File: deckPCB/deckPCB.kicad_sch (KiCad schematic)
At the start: 29 parts, among them J1 USB_C_Receptacle_USB2.0_16P, J2 Conn_01x06_Pin, SW1 SW_Push, SW10 SW_Push, SW11 SW_Push, SW12 SW_Push, SW13 SW_Push, SW14 SW_Push, SW15 SW_Push, SW2 SW_Push, SW3 SW_Push, SW4 SW_Push, SW5 SW_Push, SW6 SW_Push, SW7 SW_Push, SW8 SW_Push, SW9 SW_Push, U1 RP2040, U2 W25Q128JVE, U3 IP5306, U4 AMS1117-3.3, U5 PAM8403DR, X1 DF40HC_3.0_-100DS-0.4V_58, X2 DF40HC_3.0_-100DS-0.4V_58

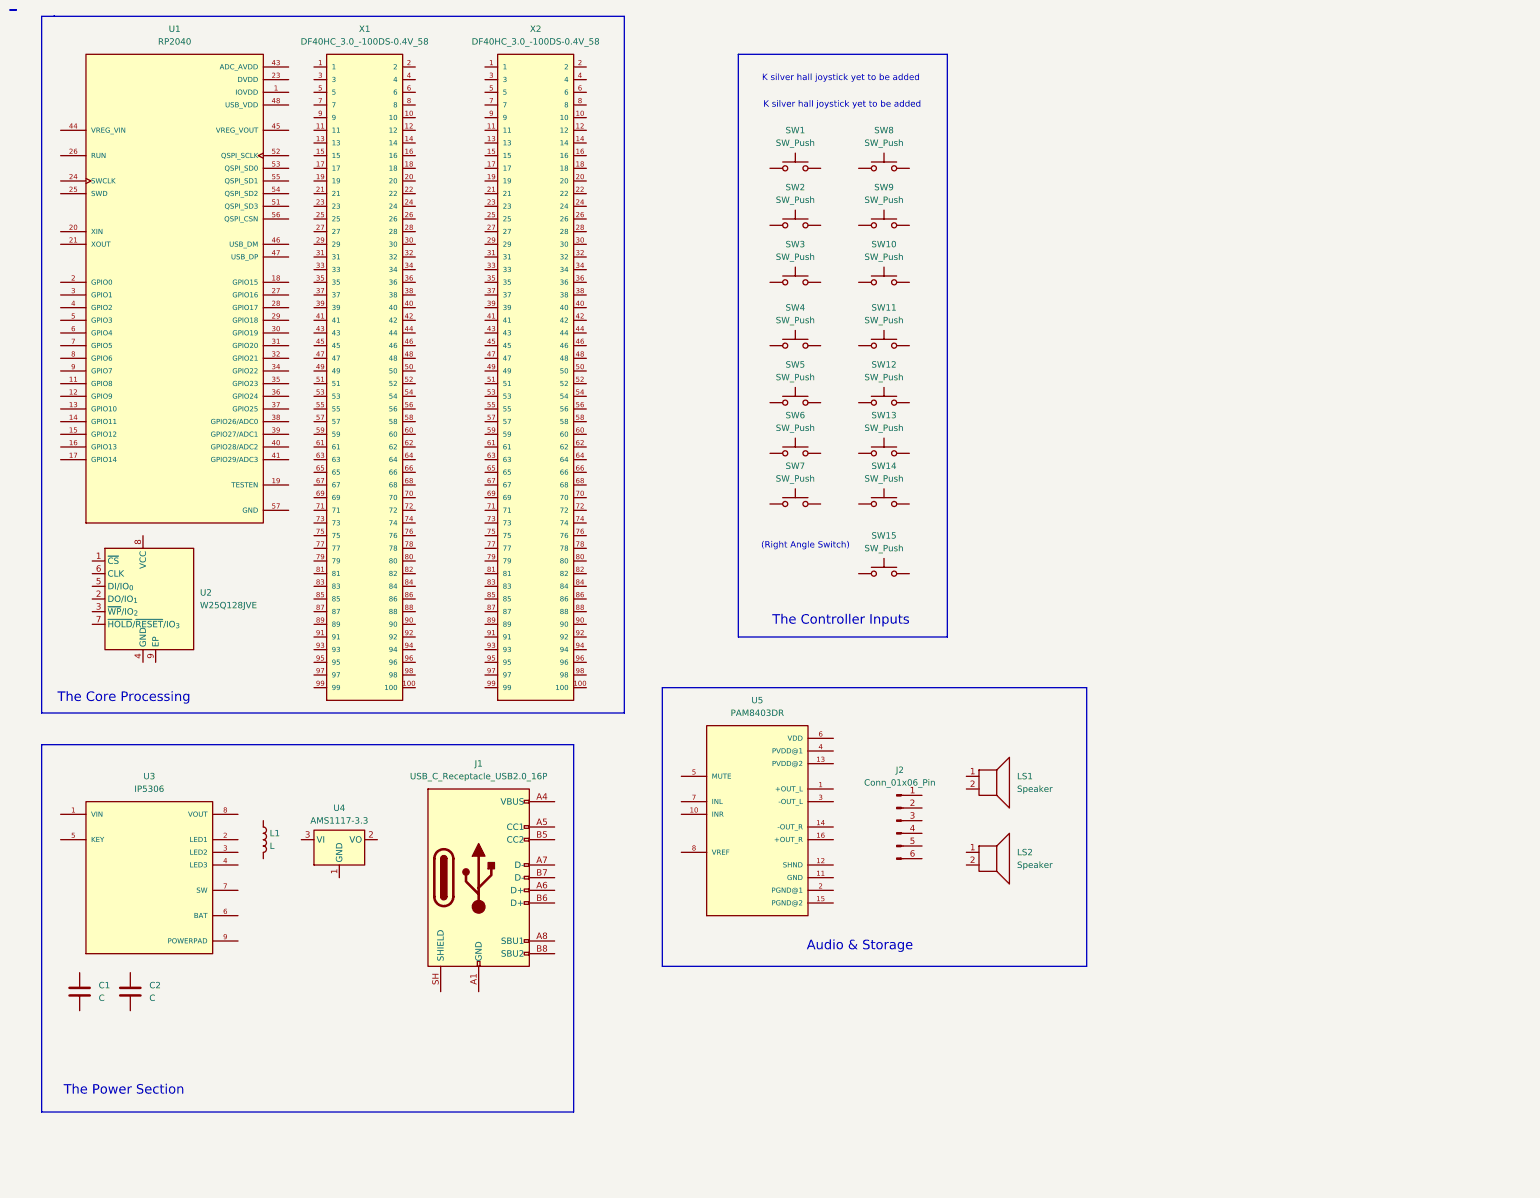
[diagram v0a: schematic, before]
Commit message: Finishing with the passives.
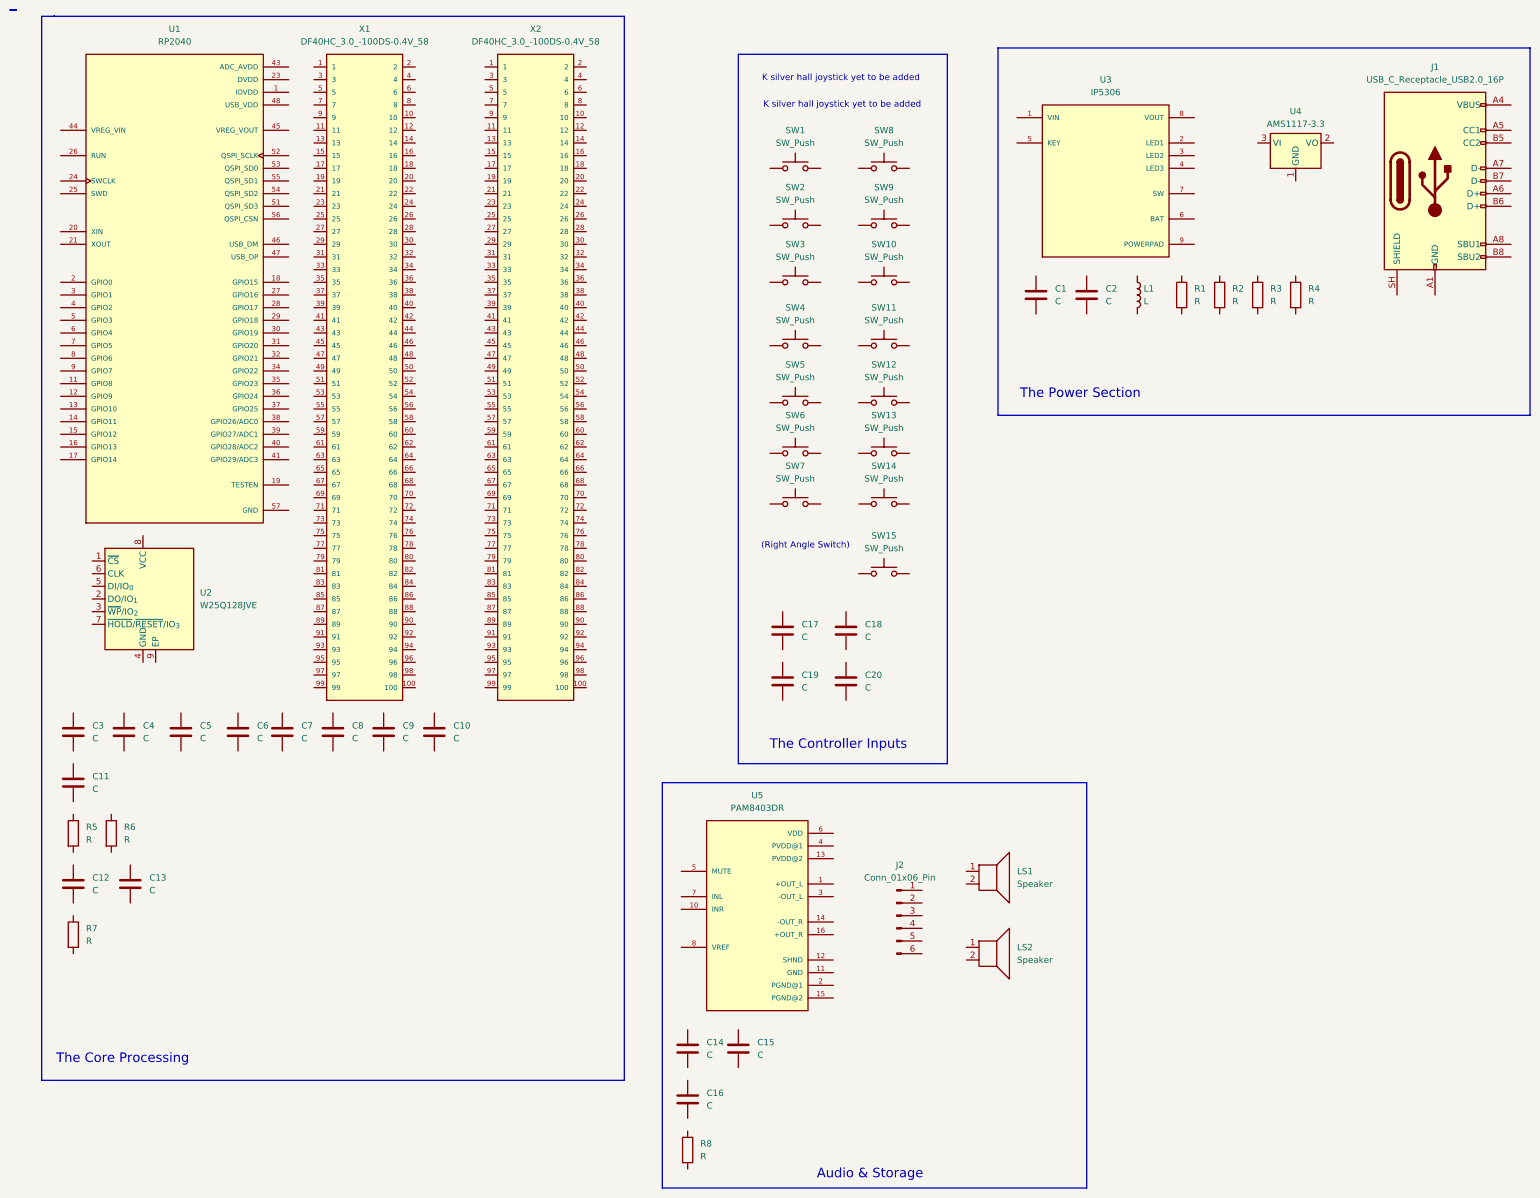
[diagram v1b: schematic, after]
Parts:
- added C10, C11, C12, C13, C14, C15, C16, C17, C18, C19, C20, C3, C4, C5, C6, C7, C8, C9: C, symbol Device:C
- added R1, R2, R3, R4, R5, R6, R7, R8: R, symbol Device:R
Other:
- moved on the sheet: C1, C2, J1, J2, L1, LS1, LS2, U3, U4, U5

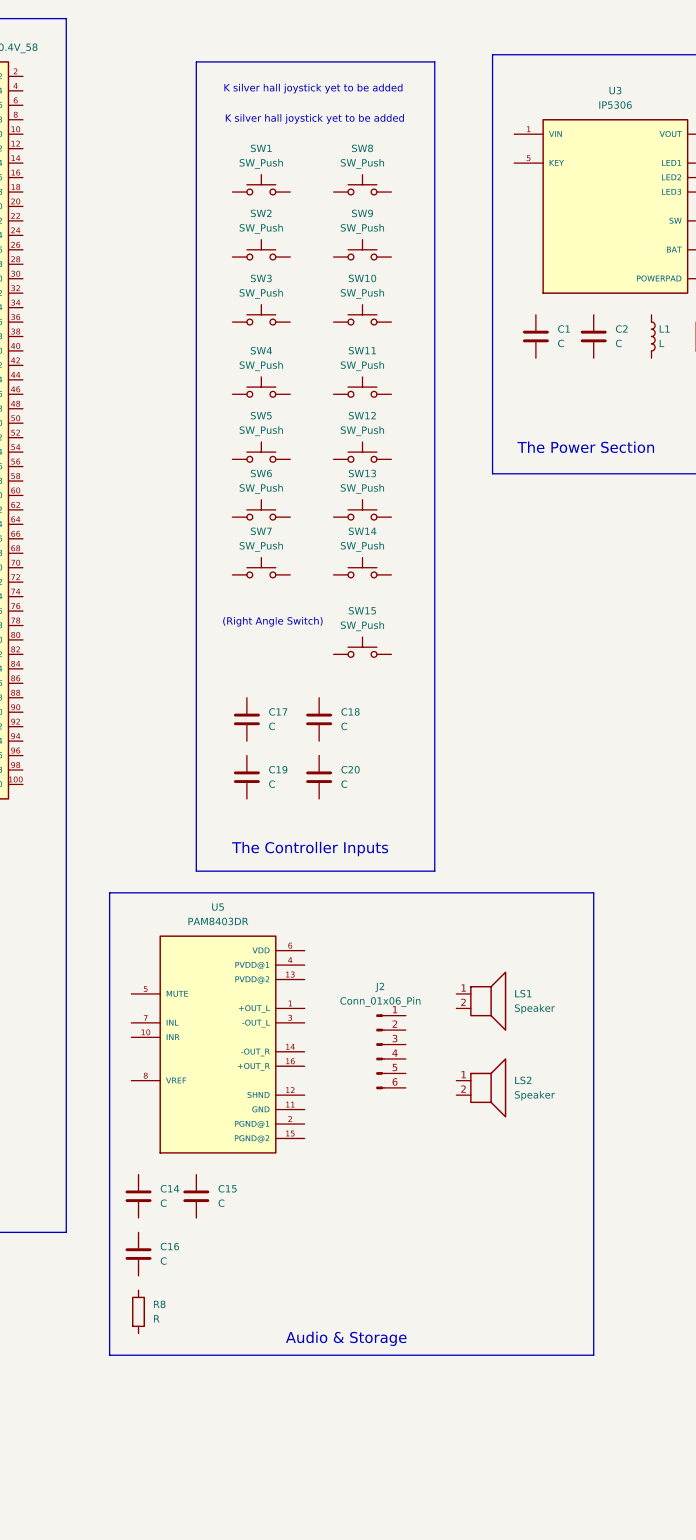
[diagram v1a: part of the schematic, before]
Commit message: hall symbol in the schematic
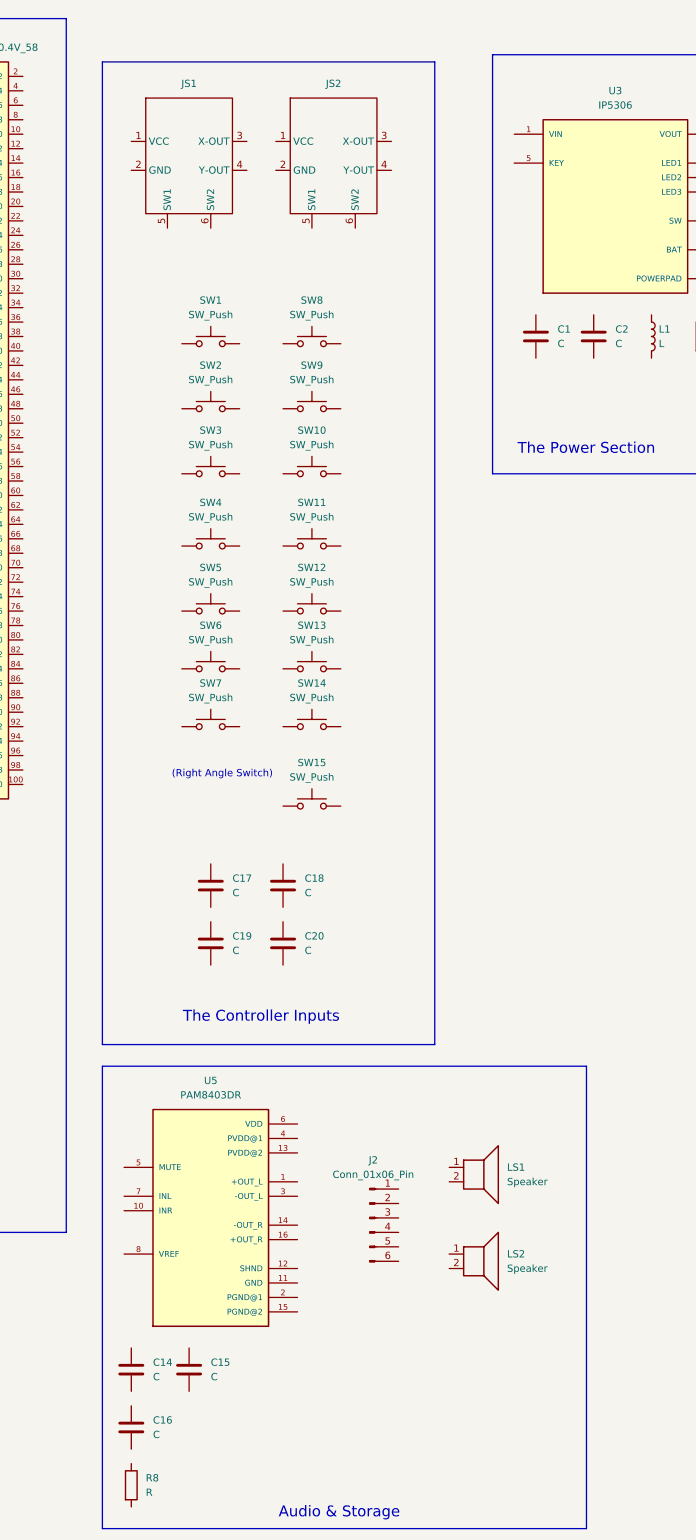
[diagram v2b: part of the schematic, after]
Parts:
- added JS1, JS2: (no value), symbol ArxDeck_Custom:K-Silver_JH16
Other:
- note removed: "K silver hall joystick yet to be added"
- moved on the sheet: C14, C15, C16, C17, C18, C19, C20, J2, LS1, LS2, R8, SW1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

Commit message: wiring_power
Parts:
- added BT1: Battery_Cell, symbol Device:Battery_Cell
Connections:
- net IOVDD is gone; now on net DVDD: U1.1 (IOVDD), U1.10 (IOVDD), U1.22 (IOVDD), U1.33 (IOVDD), U1.42 (IOVDD), U1.49 (IOVDD)
- net DVDD: now also C2.1, U1.44 (VREG_VIN), U4.2 (VO)
- net GND: now reaches J1.A1 (GND), J1.A12 (GND), J1.B1 (GND), J1.B12 (GND)
- net GND: now also U1.57 (GND), U3.9 (POWERPAD), U4.1 (GND), BT1.2 (-)
- net VBUS_5V: now reaches J1.A4 (VBUS), J1.A9 (VBUS), J1.B4 (VBUS), J1.B9 (VBUS)
- net CC1: now reaches J1.A5 (CC1)
- net CC2: now reaches J1.B5 (CC2)
- net CPC1: now reaches L1.2
- net CPC1: now also C1.1, U3.8 (VOUT)
- net BATT+: now reaches U3.6 (BAT)
- net BATT+: now also BT1.1 (+)
- net SW_NODE: now reaches U3.7 (SW)
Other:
- moved on the sheet: C1, C10, C11, C12, C13, C14, C15, C16, C17, C18, C19, C2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
